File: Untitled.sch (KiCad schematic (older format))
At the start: 28 parts, among them J1 JAMMA, J2 CONN_01X06, J5 PWR_IN, J6 DC2DC, J7 SCART-F, SW1 SW_Push, SW2 SW_Push, SW3 SW_Push, U1 LD1117S33TR, U2 ESP32-WROOM, U3 TLC5926IDW, U4 TLC5926IDW

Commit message: Lynn almost done
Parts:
- removed C1, C2, C3: 4.7u, Capacitors_SMD:C_1206_HandSoldering, symbol CP
- removed J1: JAMMA, JAMMA:JAMMA, symbol CONN_02X28
- removed J5: PWR_IN, Connectors:BARREL_JACK, symbol BARREL_JACK
- removed J6: DC2DC, NQR010A0X4Z:NQR010A0X4Z, symbol CONN_01X05
- removed J7: SCART-F, w_conn_av:SCART, symbol SCART-F
- removed R10: 100, Resistors_SMD:R_1206_HandSoldering, symbol R
- removed R3, R4: 470, Resistors_SMD:R_1206_HandSoldering, symbol R
- removed R5: 10K, Resistors_SMD:R_1206_HandSoldering, symbol R
- removed R6: 1K, Resistors_SMD:R_1206_HandSoldering, symbol R
- removed R7: 240, Resistors_SMD:R_1206_HandSoldering, symbol R
- removed R8: 500, Potentiometers:Potentiometer_Bourns_3296W_3-8Zoll_Inline_ScrewUp, symbol R_Variable
- removed R9: 33, Resistors_SMD:R_1206_HandSoldering, symbol R
- removed SW1, SW2, SW3: SW_Push, Buttons_Switches_SMD:SW_SPST_EVQPE1, symbol SW_Push
- added D1, D10, D11, D12, D13, D14, D15, D16, D17, D18, D19, D2, D20, D21, D22, D23, D24, D25, D26, D27, D28, D29, D3, D30, D31, D32, D33, D34, D35, D36, D37, D38, D39, D4, D40, D41, D42, D43, D44, D45, D46, D47, D48, D5, D6, D7, D8, D9: LED, LEDs:LED_1206_HandSoldering, symbol LED
- added J1: USB_B, Connectors:USB_Mini-B, symbol USB_B
- added U5: TLC5926IDW, Housings_SOIC:SOIC-24W_7.5x15.4mm_Pitch1.27mm, symbol TLC5926IDW
- R1: value 330 -> 10K
- R2: value 470 -> 330
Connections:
- net labels added: PROG, RESET
- net labels removed: +12V, A1, A2, B1, B2, BLUE, C1, C2, COIN1, COIN2, D1, D2, DOWN1, DOWN2, GREEN, LEFT1, LEFT2, RED, RIGHT1, RIGHT2, SERVICE, SPEAKER, START1, START2, SYNC, TEST, UP1, UP2, VIDEO_GND
- wire segments 77 -> 35
- no-connect marks 57 -> 30
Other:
- moved on the sheet: C4, J2, R11, R12, U1, U2, U3, U4

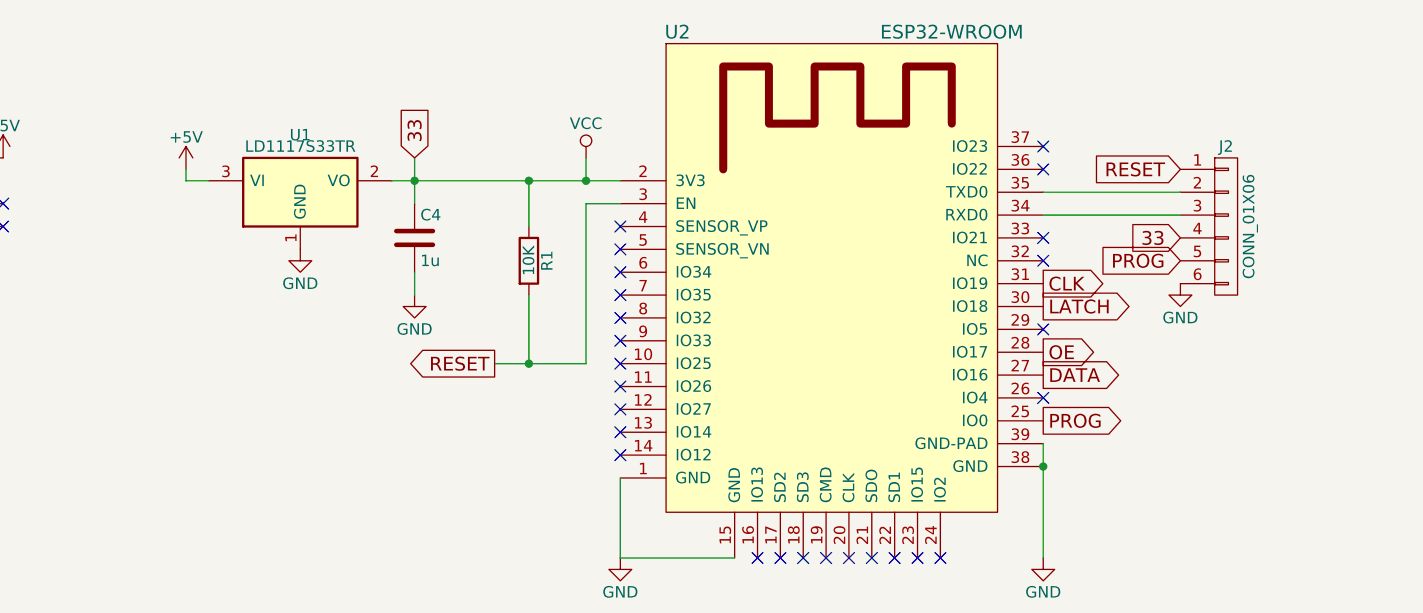
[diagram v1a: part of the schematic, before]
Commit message: Lynn V1
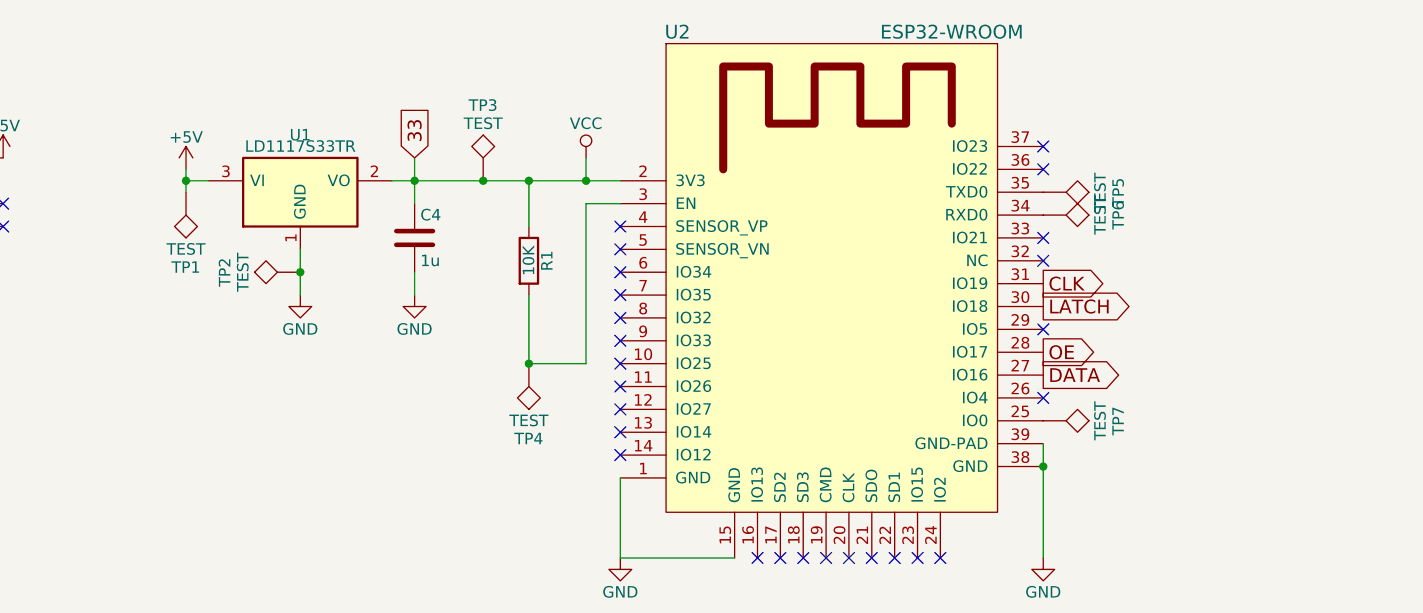
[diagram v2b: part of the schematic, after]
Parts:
- removed J2: CONN_01X06, Pin_Headers:Pin_Header_Straight_1x06, symbol CONN_01X06
- added TP1, TP3, TP4, TP5, TP6, TP7: TEST, Measurement_Points:Measurement_Point_Round-SMD-Pad_Small, symbol TEST
- added TP2: TEST, Measurement_Points:Measurement_Point_Square-SMD-Pad_Small, symbol TEST
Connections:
- net +5V: now also TP1.1
- net GND: now also TP2.1
- net VCC: now also TP3.1
- net at U2.34 (RXD0): now also TP6.1
- net at U2.35 (TXD0): now also TP5.1
- net PROG: no longer names the net of U2.25 (IO0)
- net PROG: now also TP7.1
- net RESET: no longer names the net of R1.2, U2.3 (EN)
- net RESET: now also TP4.1
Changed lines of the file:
@@
 	6050 2450 6050 2950
 Connection ~ 6050 2550
-$Comp
-L CONN_01X06 J2
-U 1 1 5A4B1405
-P 6850 1500
-F 0 "J2" H 6850 1850 50  0000 C CNN
-F 1 "CONN_01X06" V 6950 1500 50  0000 C CNN
-F 2 "Pin_Headers:Pin_Header_Straight_1x06" H 6850 1500 50  0001 C CNN
-F 3 "" H 6850 1500 50  0001 C CNN
-	1    6850 1500
-	1    0    0    -1
-$EndComp
-Wire Wire Line
-	6650 1350 6050 1350
-Wire Wire Line
-	6050 1450 6650 1450
-Text GLabel 6650 1550 0    60   Input ~ 0
-33
 Text GLabel 3300 1200 1    60   Input ~ 0
 33
@@
 L GND #PWR03
 U 1 1 5A4B2546
-P 2800 1600
-F 0 "#PWR03" H 2800 1350 50  0001 C CNN
-F 1 "GND" H 2800 1450 50  0000 C CNN
-F 2 "" H 2800 1600 50  0001 C CNN
-F 3 "" H 2800 1600 50  0001 C CNN
-	1    2800 1600
+P 2800 1800
+F 0 "#PWR03" H 2800 1550 50  0001 C CNN
+F 1 "GND" H 2800 1650 50  0000 C CNN
+F 2 "" H 2800 1800 50  0001 C CNN
+F 3 "" H 2800 1800 50  0001 C CNN
+	1    2800 1800
 	1    0    0    -1
 $EndComp
@@
 $EndComp
 Wire Wire Line
-	2300 1250 2300 1300
+	2300 1250 2300 1350
 Wire Wire Line
 	2300 1300 2400 1300
@@
 Wire Wire Line
 	900  3600 900  4550
-$Comp
-L GND #PWR09
-U 1 1 5A51FD33
-P 6650 1750
-F 0 "#PWR09" H 6650 1500 50  0001 C CNN
-F 1 "GND" H 6650 1600 50  0000 C CNN
-F 2 "" H 6650 1750 50  0001 C CNN
-F 3 "" H 6650 1750 50  0001 C CNN
-	1    6650 1750
-	1    0    0    -1
-$EndComp
 Wire Wire Line
 	4200 1400 4050 1400
 Wire Wire Line
 	4050 1400 4050 2100
-Wire Wire Line
-	4050 2100 3650 2100
 NoConn ~ 6050 1950
 $Comp
@@
 $EndComp
 $Comp
-L +5V #PWR012
+L +5V #PWR09
 U 1 1 5A70D650
 P 3050 3900
-F 0 "#PWR012" H 3050 3750 50  0001 C CNN
+F 0 "#PWR09" H 3050 3750 50  0001 C CNN
 F 1 "+5V" H 3050 4040 50  0000 C CNN
 F 2 "" H 3050 3900 50  0001 C CNN
@@
 $EndComp
 $Comp
-L +5V #PWR013
+L +5V #PWR010
 U 1 1 5A70DFBA
 P 5550 3900
-F 0 "#PWR013" H 5550 3750 50  0001 C CNN
+F 0 "#PWR010" H 5550 3750 50  0001 C CNN
 F 1 "+5V" H 5550 4040 50  0000 C CNN
 F 2 "" H 5550 3900 50  0001 C CNN
@@
 NoConn ~ 6500 4550
 $Comp
-L GND #PWR014
+L GND #PWR011
 U 1 1 5A70E335
 P 6200 5550
-F 0 "#PWR014" H 6200 5300 50  0001 C CNN
+F 0 "#PWR011" H 6200 5300 50  0001 C CNN
 F 1 "GND" H 6200 5400 50  0000 C CNN
 F 2 "" H 6200 5550 50  0001 C CNN
@@
 $EndComp
 $Comp
-L +5V #PWR015
+L +5V #PWR012
 U 1 1 5A70E3A3
 P 8000 3900
-F 0 "#PWR015" H 8000 3750 50  0001 C CNN
+F 0 "#PWR012" H 8000 3750 50  0001 C CNN
 F 1 "+5V" H 8000 4040 50  0000 C CNN
 F 2 "" H 8000 3900 50  0001 C CNN
@@
 $EndComp
 $Comp
-L +5V #PWR016
+L +5V #PWR013
 U 1 1 5A70FBE0
 P 1500 1200
-F 0 "#PWR016" H 1500 1050 50  0001 C CNN
+F 0 "#PWR013" H 1500 1050 50  0001 C CNN
 F 1 "+5V" H 1500 1340 50  0000 C CNN
 F 2 "" H 1500 1200 50  0001 C CNN
@@
 $EndComp
 $Comp
-L GND #PWR017
+L GND #PWR014
 U 1 1 5A70FCA5
 P 1200 1800
-F 0 "#PWR017" H 1200 1550 50  0001 C CNN
+F 0 "#PWR014" H 1200 1550 50  0001 C CNN
 F 1 "GND" H 1200 1650 50  0000 C CNN
 F 2 "" H 1200 1800 50  0001 C CNN
@@
 NoConn ~ 1500 1500
 NoConn ~ 1500 1400
-Text GLabel 3650 2100 0    60   Output ~ 0
-RESET
-Text GLabel 6050 2350 2    60   Output ~ 0
-PROG
-Text GLabel 6650 1650 0    60   Input ~ 0
-PROG
-Text GLabel 6650 1250 0    60   Input ~ 0
-RESET
+$Comp
+L TEST TP4
+U 1 1 5A711D73
+P 3800 2100
+F 0 "TP4" H 3800 2400 50  0000 C BNN
+F 1 "TEST" H 3800 2350 50  0000 C CNN
+F 2 "Measurement_Points:Measurement_Point_Round-SMD-Pad_Small" H 3800 2100 50  0001 C CNN
+F 3 "" H 3800 2100 50  0001 C CNN
+	1    3800 2100
+	-1   0    0    1
+$EndComp
+$Comp
+L TEST TP3
+U 1 1 5A711E9C
+P 3600 1300
+F 0 "TP3" H 3600 1600 50  0000 C BNN
+F 1 "TEST" H 3600 1550 50  0000 C CNN
+F 2 "Measurement_Points:Measurement_Point_Round-SMD-Pad_Small" H 3600 1300 50  0001 C CNN
+F 3 "" H 3600 1300 50  0001 C CNN
+	1    3600 1300
+	1    0    0    -1
+$EndComp
+Connection ~ 3600 1300
+$Comp
+L TEST TP7
+U 1 1 5A7124CD
+P 6050 2350
+F 0 "TP7" H 6050 2650 50  0000 C BNN
+F 1 "TEST" H 6050 2600 50  0000 C CNN
+F 2 "Measurement_Points:Measurement_Point_Round-SMD-Pad_Small" H 6050 2350 50  0001 C CNN
+F 3 "" H 6050 2350 50  0001 C CNN
+	1    6050 2350
+	0    1    1    0
+$EndComp
+$Comp
+L TEST TP5
+U 1 1 5A712804
+P 6050 1350
+F 0 "TP5" H 6050 1650 50  0000 C BNN
+F 1 "TEST" H 6050 1600 50  0000 C CNN
+F 2 "Measurement_Points:Measurement_Point_Round-SMD-Pad_Small" H 6050 1350 50  0001 C CNN
+F 3 "" H 6050 1350 50  0001 C CNN
+	1    6050 1350
+	0    1    1    0
+$EndComp
+$Comp
+L TEST TP6
+U 1 1 5A7128F6
+P 6050 1450
+F 0 "TP6" H 6050 1750 50  0000 C BNN
+F 1 "TEST" H 6050 1700 50  0000 C CNN
+F 2 "Measurement_Points:Measurement_Point_Round-SMD-Pad_Small" H 6050 1450 50  0001 C CNN
+F 3 "" H 6050 1450 50  0001 C CNN
+	1    6050 1450
+	0    1    1    0
+$EndComp
+Wire Wire Line
+	3800 2100 4050 2100
+$Comp
+L TEST TP2
+U 1 1 5A712D9E
+P 2800 1700
+F 0 "TP2" H 2800 2000 50  0000 C BNN
+F 1 "TEST" H 2800 1950 50  0000 C CNN
+F 2 "Measurement_Points:Measurement_Point_Square-SMD-Pad_Small" H 2800 1700 50  0001 C CNN
+F 3 "" H 2800 1700 50  0001 C CNN
+	1    2800 1700
+	0    -1   -1   0
+$EndComp
+Wire Wire Line
+	2800 1600 2800 1800
+Connection ~ 2800 1700
+$Comp
+L TEST TP1
+U 1 1 5A712FBB
+P 2300 1350
+F 0 "TP1" H 2300 1650 50  0000 C BNN
+F 1 "TEST" H 2300 1600 50  0000 C CNN
+F 2 "Measurement_Points:Measurement_Point_Round-SMD-Pad_Small" H 2300 1350 50  0001 C CNN
+F 3 "" H 2300 1350 50  0001 C CNN
+	1    2300 1350
+	-1   0    0    1
+$EndComp
+Connection ~ 2300 1300
 $EndSCHEMATC
